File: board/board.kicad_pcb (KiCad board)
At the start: 2 copper layers, 21 x 13 mm, 1 part

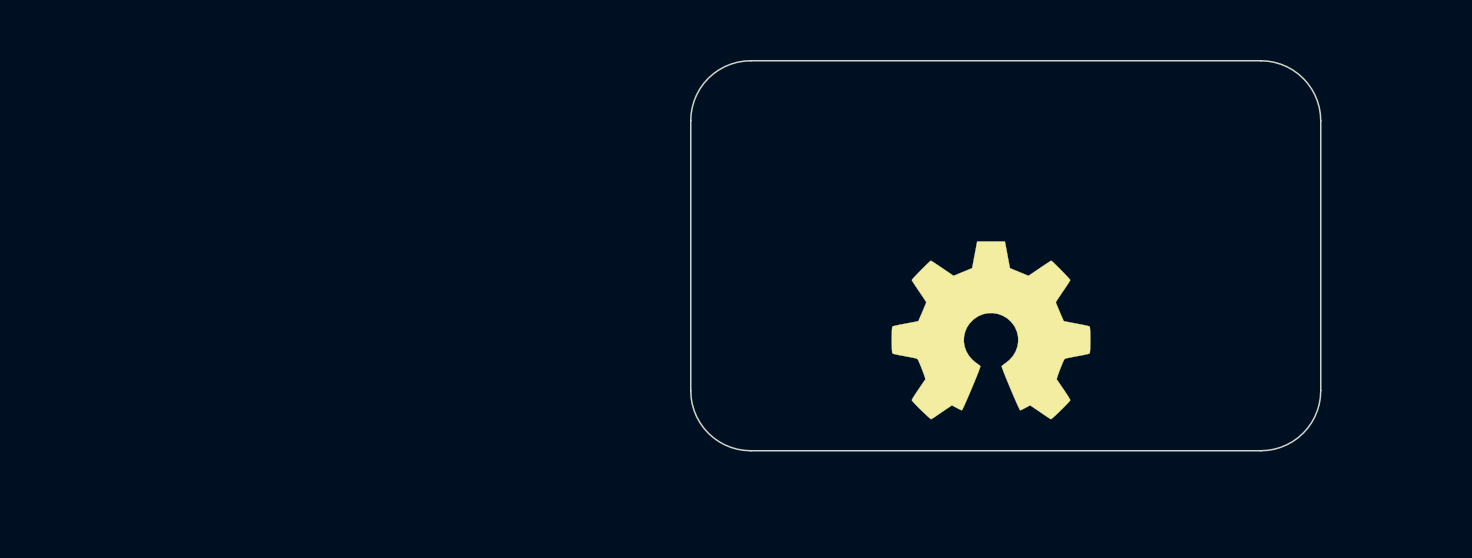
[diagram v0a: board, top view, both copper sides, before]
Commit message: initial
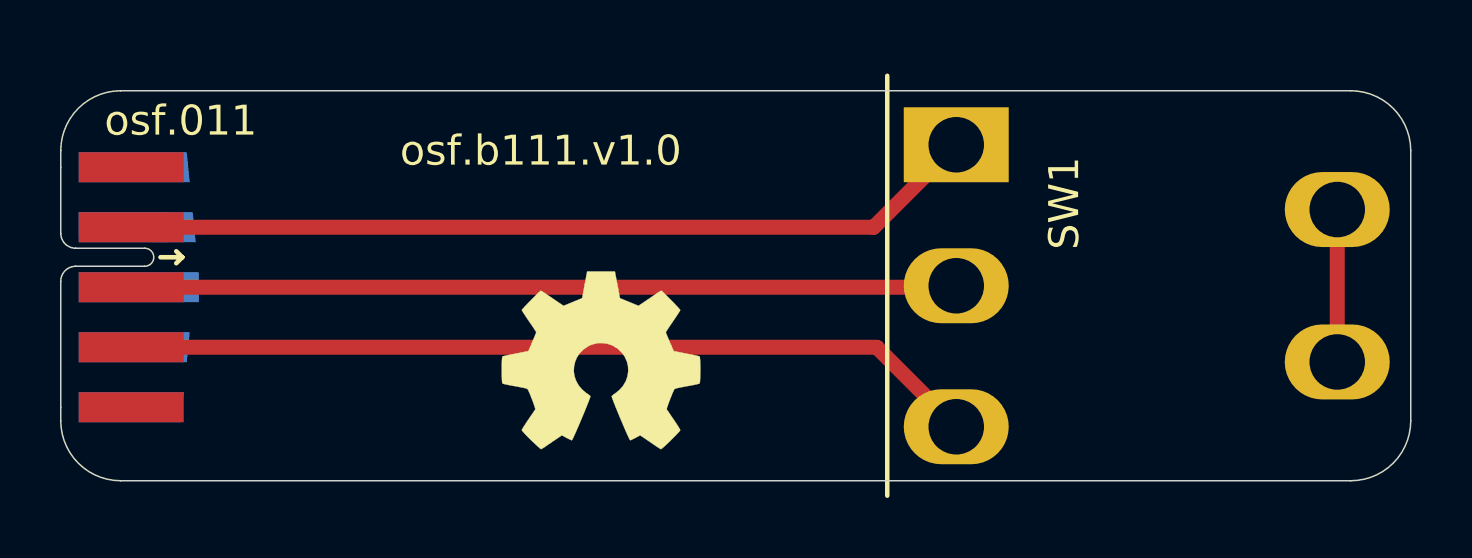
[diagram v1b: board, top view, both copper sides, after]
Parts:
- added J1: 011_GPIO, on_edge:on_edge_2x05_device, F.Cu at (119.0, 97.5)
- added SW1: SW_SPDT, b111:SW_CuK_E103MD1ABE_SPDT_Angled, F.Cu at (148.8, 97.5)
- moved LOGO1 13.0 mm to (137.0, 100.0)
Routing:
- net /switch/1: track 0.00 -> 28.6 mm
- net /switch/2: track 0.00 -> 28.6 mm
- net /switch/P: track 0.00 -> 27.5 mm
- net Net-(SW1-PadS1): track 0.00 -> 5.08 mm
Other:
- board size 21 x 13 mm -> 45 x 13 mm
- board text added: "osf.011"
- board text added: "osf.b111.v1.0"
